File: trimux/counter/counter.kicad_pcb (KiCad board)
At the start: 2 copper layers, 50 x 50 mm, 33 parts, among them P1 CONN_01X03, P2 CONN_01X03, P3 CONN_01X02, P4 CONN_01X03, P5 CONN_01X03, U1 trimux, U2 trimux, U3 trimux, U4 trimux, U5 trimux

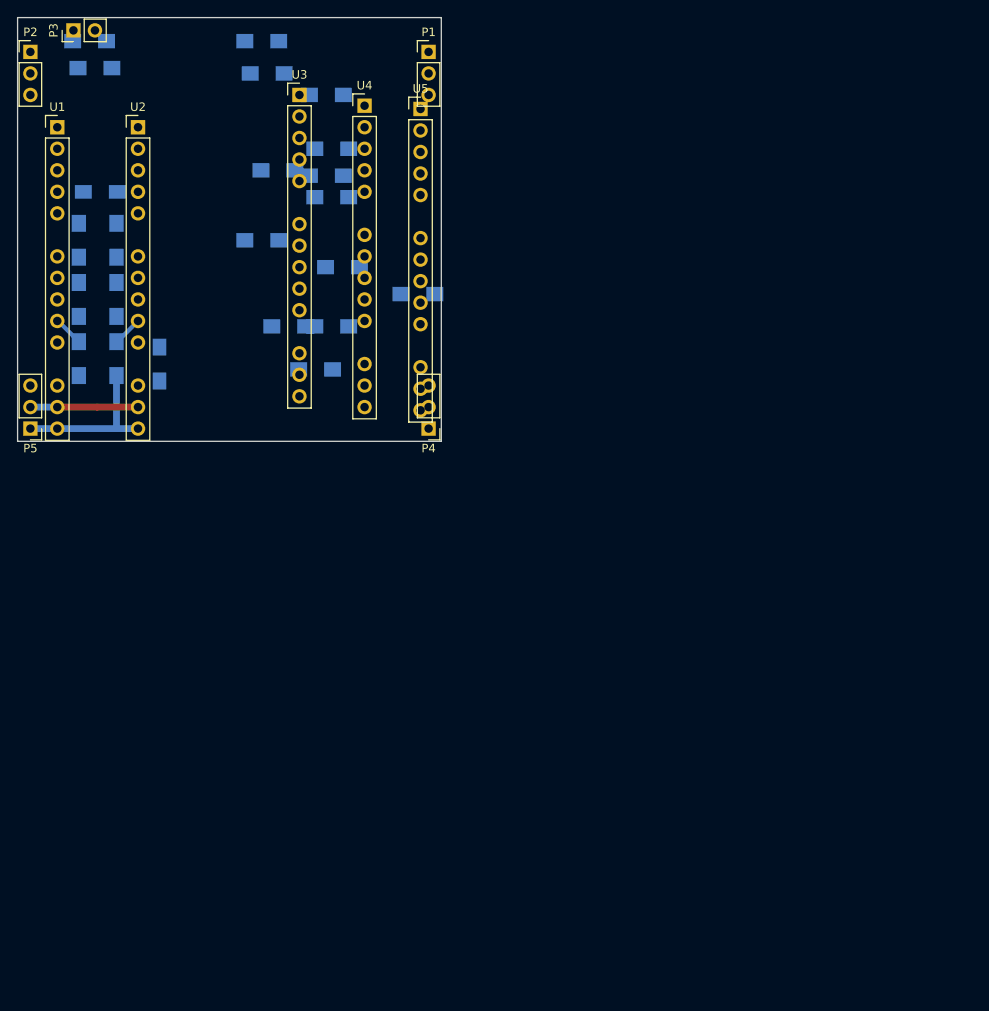
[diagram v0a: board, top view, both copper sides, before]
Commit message: counter board
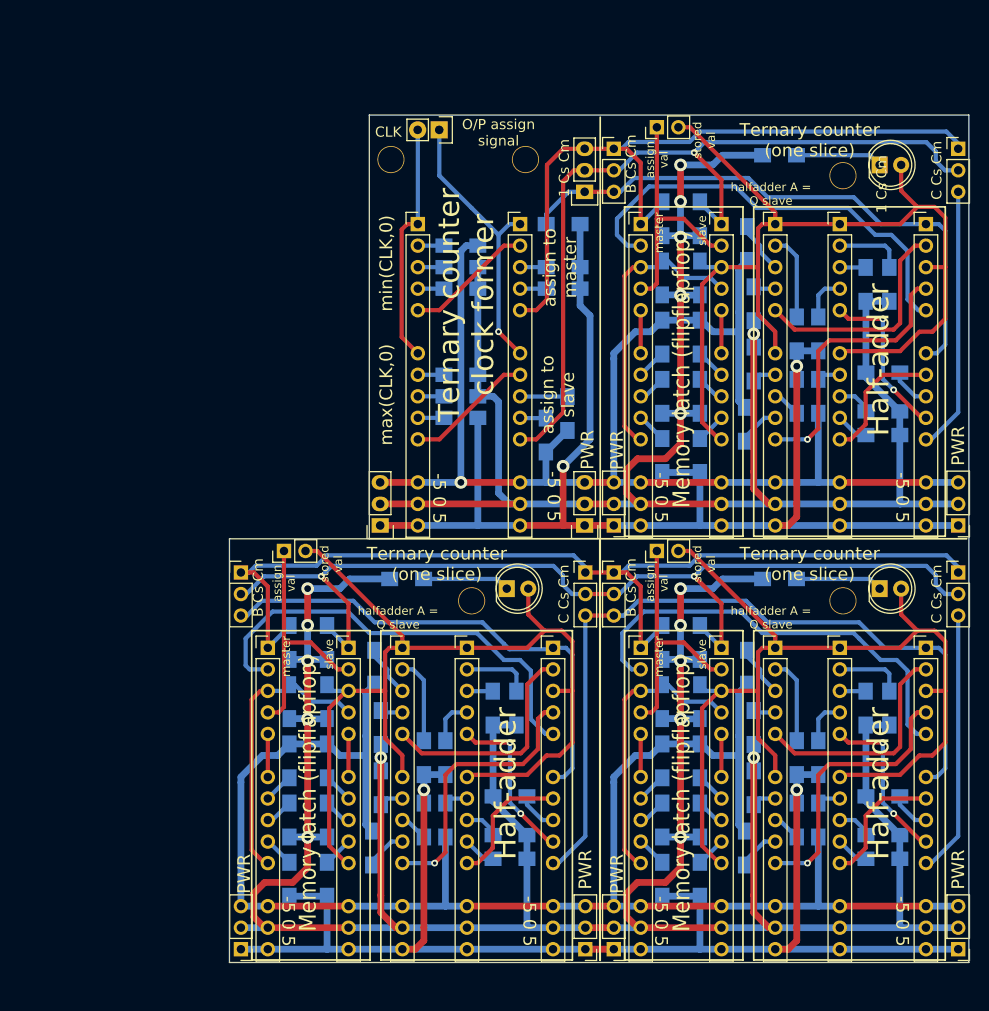
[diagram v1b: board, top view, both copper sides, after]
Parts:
- added C1: 100nF, Capacitors_SMD:C_1206_HandSoldering, B.Cu at (47.1, 95.7)
- added C1: 100nF, Capacitors_SMD:C_1206_HandSoldering, B.Cu at (91.1, 95.7)
- added C2: 100nF, Capacitors_SMD:C_1206_HandSoldering, B.Cu at (51.5, 95.7)
- added C2: 100nF, Capacitors_SMD:C_1206_HandSoldering, B.Cu at (95.5, 95.7)
- added D1: LED_Dual_2pin, LEDs:LED-5MM, F.Cu at (72.7, 82.4)
- added D1: LED_Dual_2pin, LEDs:LED-5MM, F.Cu at (116.7, 82.4)
- added D1: LED_Dual_2pin, LEDs:LED-5MM, F.Cu at (116.7, 32.4)
- added P1: CONN_01X03, Pin_Headers:Pin_Header_Straight_1x03_Pitch2.54mm, F.Cu at (82.0, 80.5)
- added P1: CONN_01X03, Pin_Headers:Pin_Header_Straight_1x03_Pitch2.54mm, F.Cu at (126.0, 80.5)
- added P2: CONN_01X03, Pin_Headers:Pin_Header_Straight_1x03_Pitch2.54mm, F.Cu at (41.4, 80.5)
- added P2: CONN_01X03, Pin_Headers:Pin_Header_Straight_1x03_Pitch2.54mm, F.Cu at (85.4, 80.5)
- added P3: CONN_01X02, Pin_Headers:Pin_Header_Straight_1x02_Pitch2.54mm, F.Cu at (46.4, 77.9)
- added P3: CONN_01X02, Pin_Headers:Pin_Header_Straight_1x02_Pitch2.54mm, F.Cu at (90.4, 77.9)
- added P4: CONN_01X03, Pin_Headers:Pin_Header_Straight_1x03_Pitch2.54mm, F.Cu at (82.0, 124.9)
- added P4: CONN_01X03, Pin_Headers:Pin_Header_Straight_1x03_Pitch2.54mm, F.Cu at (126.0, 124.9)
- added P5: CONN_01X03, Pin_Headers:Pin_Header_Straight_1x03_Pitch2.54mm, F.Cu at (41.4, 124.9)
- added P5: CONN_01X03, Pin_Headers:Pin_Header_Straight_1x03_Pitch2.54mm, F.Cu at (85.4, 124.9)
- added P6: CONN_01X02, Pin_Headers:Pin_Header_Straight_1x02, F.Cu at (64.8, 28.2)
- added P7: CONN_01X03, Pin_Headers:Pin_Header_Straight_1x03, F.Cu at (81.9, 35.6)
- added P8: CONN_01X03, Pin_Headers:Pin_Header_Straight_1x03, F.Cu at (81.9, 74.9)
- added P9: CONN_01X03, Pin_Headers:Pin_Header_Straight_1x03, F.Cu at (57.8, 74.9)
- added R1: 10k, Resistors_SMD:R_1206_HandSoldering, B.Cu at (51.5, 88.7)
- added R1: 10k, Resistors_SMD:R_1206_HandSoldering, B.Cu at (95.5, 88.7)
- added R10: 150, Resistors_SMD:R_1206_HandSoldering, B.Cu at (73.9, 96.5)
- added R10: 150, Resistors_SMD:R_1206_HandSoldering, B.Cu at (117.9, 96.5)
- added R11: 150, Resistors_SMD:R_1206_HandSoldering, B.Cu at (57.1, 91.7)
- added R11: 150, Resistors_SMD:R_1206_HandSoldering, B.Cu at (101.1, 91.7)
- added R12: 150, Resistors_SMD:R_1206_HandSoldering, B.Cu at (71.1, 96.5)
- added R12: 150, Resistors_SMD:R_1206_HandSoldering, B.Cu at (115.1, 96.5)
- added R13: 150, Resistors_SMD:R_1206_HandSoldering, B.Cu at (57.9, 98.8)
- added R13: 150, Resistors_SMD:R_1206_HandSoldering, B.Cu at (101.9, 98.8)
- added R14: 150, Resistors_SMD:R_1206_HandSoldering, B.Cu at (65.5, 102.3)
- added R14: 150, Resistors_SMD:R_1206_HandSoldering, B.Cu at (109.5, 102.3)
- added R15: 150, Resistors_SMD:R_1206_HandSoldering, B.Cu at (57.9, 105.9)
- added R15: 150, Resistors_SMD:R_1206_HandSoldering, B.Cu at (101.9, 105.9)
- added R16: 150, Resistors_SMD:R_1206_HandSoldering, B.Cu at (65.5, 109.7)
- added R16: 150, Resistors_SMD:R_1206_HandSoldering, B.Cu at (109.5, 109.7)
- added R17: 150, Resistors_SMD:R_1206_HandSoldering, B.Cu at (62.9, 109.7)
- added R17: 150, Resistors_SMD:R_1206_HandSoldering, B.Cu at (106.9, 109.7)
- added R18: 150, Resistors_SMD:R_1206_HandSoldering, B.Cu at (73.1, 111.5)
- added R18: 150, Resistors_SMD:R_1206_HandSoldering, B.Cu at (117.1, 111.5)
- added R19: 150, Resistors_SMD:R_1206_HandSoldering, B.Cu at (56.8, 113.0)
- added R19: 150, Resistors_SMD:R_1206_HandSoldering, B.Cu at (100.8, 113.0)
- added R2: 10k, Resistors_SMD:R_1206_HandSoldering, B.Cu at (47.1, 88.7)
- added R2: 10k, Resistors_SMD:R_1206_HandSoldering, B.Cu at (91.1, 88.7)
- added R20: 150, Resistors_SMD:R_1206_HandSoldering, B.Cu at (73.1, 114.3)
- added R20: 150, Resistors_SMD:R_1206_HandSoldering, B.Cu at (117.1, 114.3)
- added R21: 150, Resistors_SMD:R_1206_HandSoldering, B.Cu at (73.1, 106.9)
- added R21: 150, Resistors_SMD:R_1206_HandSoldering, B.Cu at (117.1, 106.9)
- added R22: 1k, Resistors_SMD:R_1206_HandSoldering, B.Cu at (60.9, 81.2)
- added R22: 1k, Resistors_SMD:R_1206_HandSoldering, B.Cu at (104.9, 81.2)
- added R22: 1k, Resistors_SMD:R_1206_HandSoldering, B.Cu at (104.9, 31.2)
- added R23: 150, Resistors_SMD:R_1206_HandSoldering, B.Cu at (67.3, 41.9)
- added R24: 150, Resistors_SMD:R_1206_HandSoldering, B.Cu at (67.3, 44.5)
- added R25: 150, Resistors_SMD:R_1206_HandSoldering, B.Cu at (79.4, 44.5)
- added R26: 150, Resistors_SMD:R_1206_HandSoldering, B.Cu at (67.3, 47.0)
- added R27: 150, Resistors_SMD:R_1206_HandSoldering, B.Cu at (79.4, 47.0)
- added R28: 150, Resistors_SMD:R_1206_HandSoldering, B.Cu at (67.3, 57.1)
- added R29: 150, Resistors_SMD:R_1206_HandSoldering, B.Cu at (67.3, 59.7)
- added R3: 150, Resistors_SMD:R_1206_HandSoldering, B.Cu at (47.1, 102.7)
- added R3: 150, Resistors_SMD:R_1206_HandSoldering, B.Cu at (91.1, 102.7)
- added R30: 150, Resistors_SMD:R_1206_HandSoldering, B.Cu at (79.9, 61.7)
- added R31: 150, Resistors_SMD:R_1206_HandSoldering, B.Cu at (67.3, 62.2)
- added R32: 150, Resistors_SMD:R_1206_HandSoldering, B.Cu at (77.3, 64.3)
- added R33: 150, Resistors_SMD:R_1206_HandSoldering, B.Cu at (79.4, 39.4)
- added R4: 150, Resistors_SMD:R_1206_HandSoldering, B.Cu at (51.5, 102.7)
- added R4: 150, Resistors_SMD:R_1206_HandSoldering, B.Cu at (95.5, 102.7)
- added R5: 150, Resistors_SMD:R_1206_HandSoldering, B.Cu at (47.1, 109.7)
- added R5: 150, Resistors_SMD:R_1206_HandSoldering, B.Cu at (91.1, 109.7)
- added R6: 150, Resistors_SMD:R_1206_HandSoldering, B.Cu at (51.5, 109.7)
- added R6: 150, Resistors_SMD:R_1206_HandSoldering, B.Cu at (95.5, 109.7)
- added R7: 150, Resistors_SMD:R_1206_HandSoldering, B.Cu at (47.1, 116.7)
- added R7: 150, Resistors_SMD:R_1206_HandSoldering, B.Cu at (91.1, 116.7)
- added R8: 150, Resistors_SMD:R_1206_HandSoldering, B.Cu at (51.5, 116.7)
- added R8: 150, Resistors_SMD:R_1206_HandSoldering, B.Cu at (95.5, 116.7)
- added R9: 150, Resistors_SMD:R_1206_HandSoldering, B.Cu at (62.9, 102.3)
- added R9: 150, Resistors_SMD:R_1206_HandSoldering, B.Cu at (106.9, 102.3)
- added REF**: SolderWirePad_single_2-5mmDrill, Wire_Pads:SolderWirePad_single_2-5mmDrill, F.Cu at (112.4, 83.8)
- added REF**: SolderWirePad_single_2-5mmDrill, Wire_Pads:SolderWirePad_single_2-5mmDrill, F.Cu at (68.6, 83.8)
- added REF**: SolderWirePad_single_2-5mmDrill, Wire_Pads:SolderWirePad_single_2-5mmDrill, F.Cu at (112.4, 33.7)
- added REF**: SolderWirePad_single_2-5mmDrill, Wire_Pads:SolderWirePad_single_2-5mmDrill, F.Cu at (59.1, 31.8)
- added REF**: SolderWirePad_single_2-5mmDrill, Wire_Pads:SolderWirePad_single_2-5mmDrill, F.Cu at (74.9, 31.8)
- added U1: trimux, trimux:trimux1x15_2.54, F.Cu at (44.5, 89.4)
- added U1: trimux, trimux:trimux1x15_2.54, F.Cu at (88.5, 89.4)
- added U2: trimux, trimux:trimux1x15_2.54, F.Cu at (54.1, 89.4)
- added U2: trimux, trimux:trimux1x15_2.54, F.Cu at (98.1, 89.4)
- added U3: trimux, trimux:trimux1x15_2.54, F.Cu at (60.4, 89.4)
- added U3: trimux, trimux:trimux1x15_2.54, F.Cu at (104.4, 89.4)
- added U4: trimux, trimux:trimux1x15_2.54, F.Cu at (68.0, 89.4)
- added U4: trimux, trimux:trimux1x15_2.54, F.Cu at (112.0, 89.4)
- added U5: trimux, trimux:trimux1x15_2.54, F.Cu at (78.2, 89.4)
- added U5: trimux, trimux:trimux1x15_2.54, F.Cu at (122.2, 89.4)
- added U6: trimux, trimux:trimux1x15_2.54, F.Cu at (62.2, 39.4)
- added U7: trimux, trimux:trimux1x15_2.54, F.Cu at (74.3, 39.4)
- moved R1 73.6 mm to (95.5, 38.7), turned to 270 degrees
- moved R9 72.0 mm to (106.9, 52.3), turned to 270 degrees
- moved R2 70.7 mm to (91.1, 38.7), turned to 270 degrees
- moved R10 70.1 mm to (117.9, 46.5), turned to 270 degrees
- moved R3 69.8 mm to (91.1, 52.7)
- moved R4 69.8 mm to (95.5, 52.7)
- moved R5 69.8 mm to (91.1, 59.7)
- moved R6 69.8 mm to (95.5, 59.7)
- moved R7 69.8 mm to (91.1, 66.7)
- moved R8 69.8 mm to (95.5, 66.7)
- moved U1 69.8 mm to (88.5, 39.4)
- moved U2 69.8 mm to (98.1, 39.4)
- moved P2 69.8 mm to (85.4, 30.5)
- moved P3 69.8 mm to (90.4, 27.9)
- moved P5 69.8 mm to (85.4, 74.9)
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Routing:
- net GNDREF: track 12.7 -> 552.1 mm, vias 0 -> 18
- net -5V: track 0.00 -> 368.3 mm, vias 0 -> 1
- net /A: track 0.00 -> 362.6 mm
- net +5V: track 19.0 -> 315.0 mm, vias 0 -> 4
- net /Cs: track 0.00 -> 216.1 mm, vias 0 -> 3
- net /Cm: track 0.00 -> 204.1 mm
- net /B: track 0.00 -> 187.7 mm
- net /Am: track 0.00 -> 158.0 mm
- net /Bs: track 0.00 -> 101.5 mm
- net /A+1: track 0.00 -> 97.8 mm, vias 0 -> 3
- net /C: track 0.00 -> 96.8 mm
- net /BmAs: track 0.00 -> 88.6 mm
- net /A-1: track 0.00 -> 81.4 mm
- net /max(A,0): track 0.00 -> 58.8 mm, vias 0 -> 6
- net /min(A,0): track 0.00 -> 46.6 mm
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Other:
- board size 50 x 50 mm -> 87.2 x 100 mm
- net class Default: via_drill 0.5 -> 0.4
- net class PWR: via_dia 1.2 -> 1.5
- board text added: "-5 0 5"
- board text added: "1 Cs Cm"
- board text added: "B Cs Cm"
- board text added: "C Cs Cm"
- board text added: "CLK"
- board text added: "Half-adder"
- board text added: "Memory latch (flipflapflop)"
- board text added: "O/P assign signal"
- board text added: "PWR"
- board text added: "Ternary counter (one slice)"
- board text added: "Ternary counter clock former"
- board text added: "assign to master"
- board text added: "assign to slave"
- board text added: "assign val"
- board text added: "halfadder A = Q slave"
- board text added: "master"
- board text added: "max(CLK,0)"
- board text added: "min(CLK,0)"
- board text added: "slave"
- board text added: "stored val"
